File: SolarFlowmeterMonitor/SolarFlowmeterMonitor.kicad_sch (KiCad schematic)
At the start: 18 parts, among them J1 FlowMeter, J2 SP-pins, J3 Conn_01x10_Pin, J4 Solar Panel 280mA@18V, Q1 AO3413, Q2 2N7000, U1 StepDown_LM2596, U2 XL6009, U3 LoadSharing, U4 LiCharger, U7 XC6206P332MR

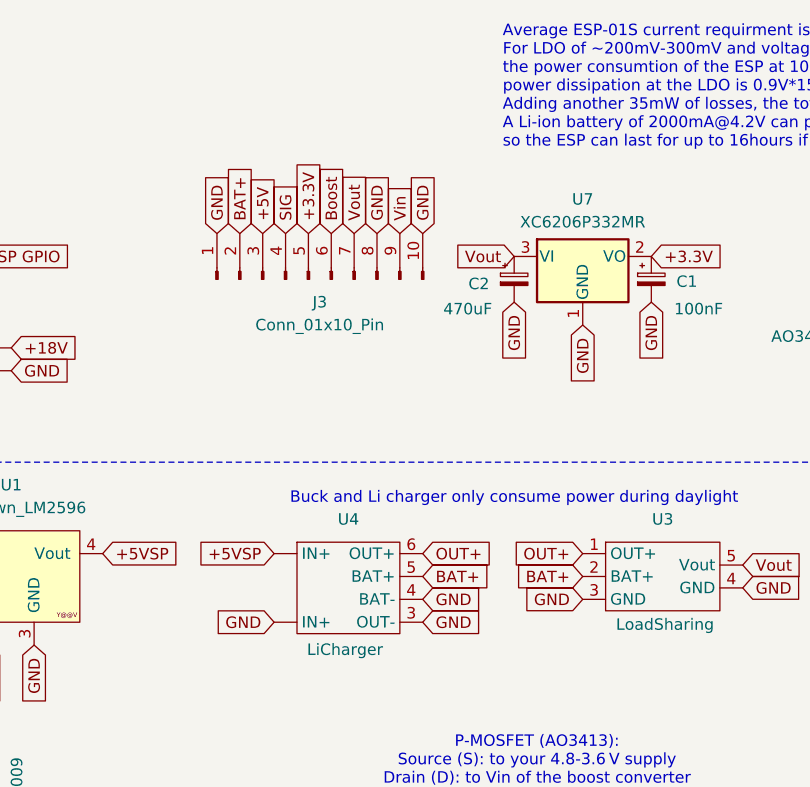
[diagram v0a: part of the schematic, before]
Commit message: fixes
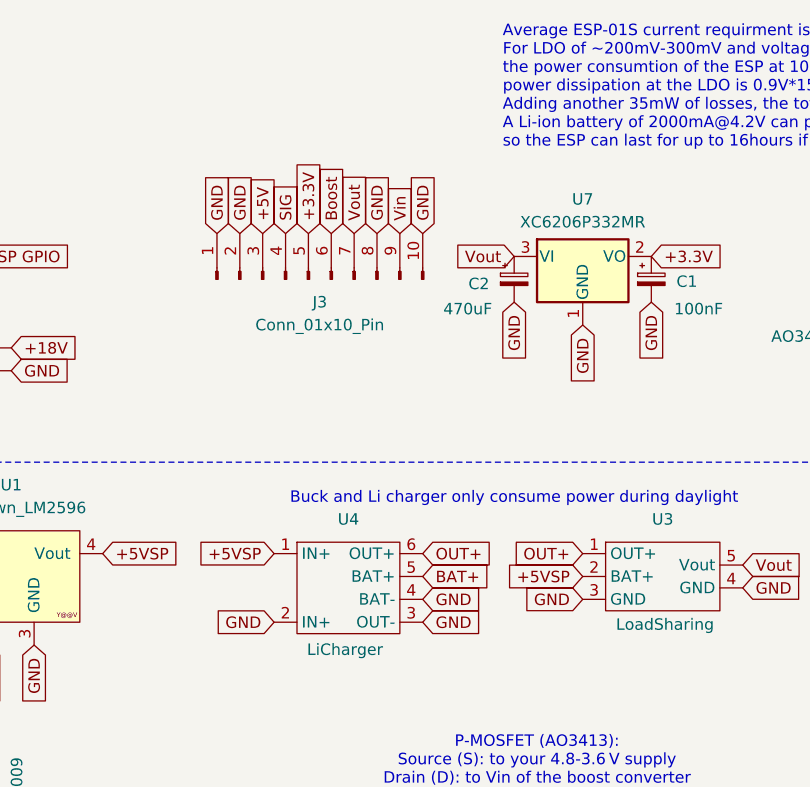
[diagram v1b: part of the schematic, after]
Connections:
- net +5VSP: now also U3.2 (BAT+), U4.1 (IN+); no longer U4. (IN+)
- net BAT+: no longer J3.2 (Pin_2), U3.2 (BAT+)
- net GND: now also J3.2 (Pin_2), U4.2 (IN+); no longer U4. (IN+)
